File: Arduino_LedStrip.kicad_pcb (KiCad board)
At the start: 2 copper layers, 52 x 71 mm, 26 parts, among them J1 Conn_L, J2 Conn_R, J3 LED0, J4 LED1, J5 LED_WS2812B, J6 Barrel_Jack, Q1 IRFZ44N, Q2 IRFZ44N, Q3 IRFZ44N, Q4 IRFZ44N, Q5 IRFZ44N, Q6 IRFZ44N, SW1 SW_Push, SW2 SW_Push, U1 TSOP4838

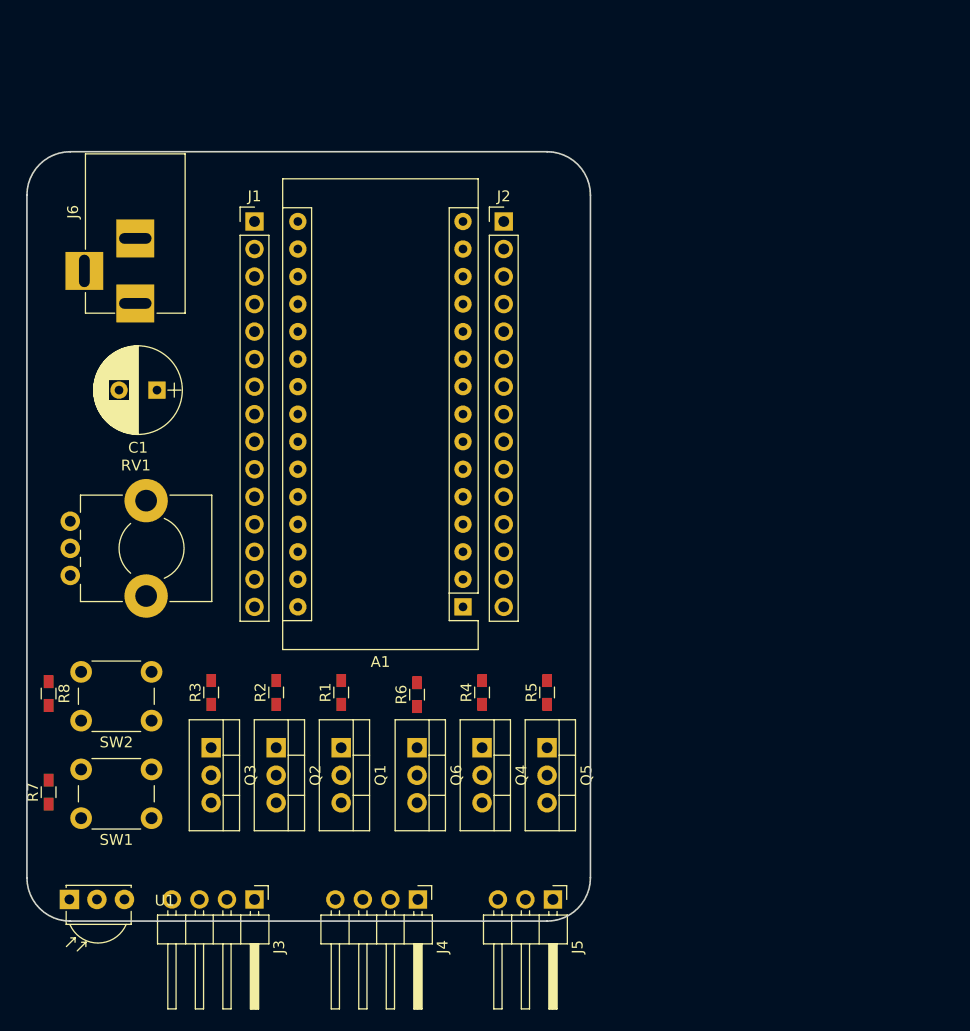
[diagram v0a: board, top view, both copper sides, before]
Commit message: Routing PCB
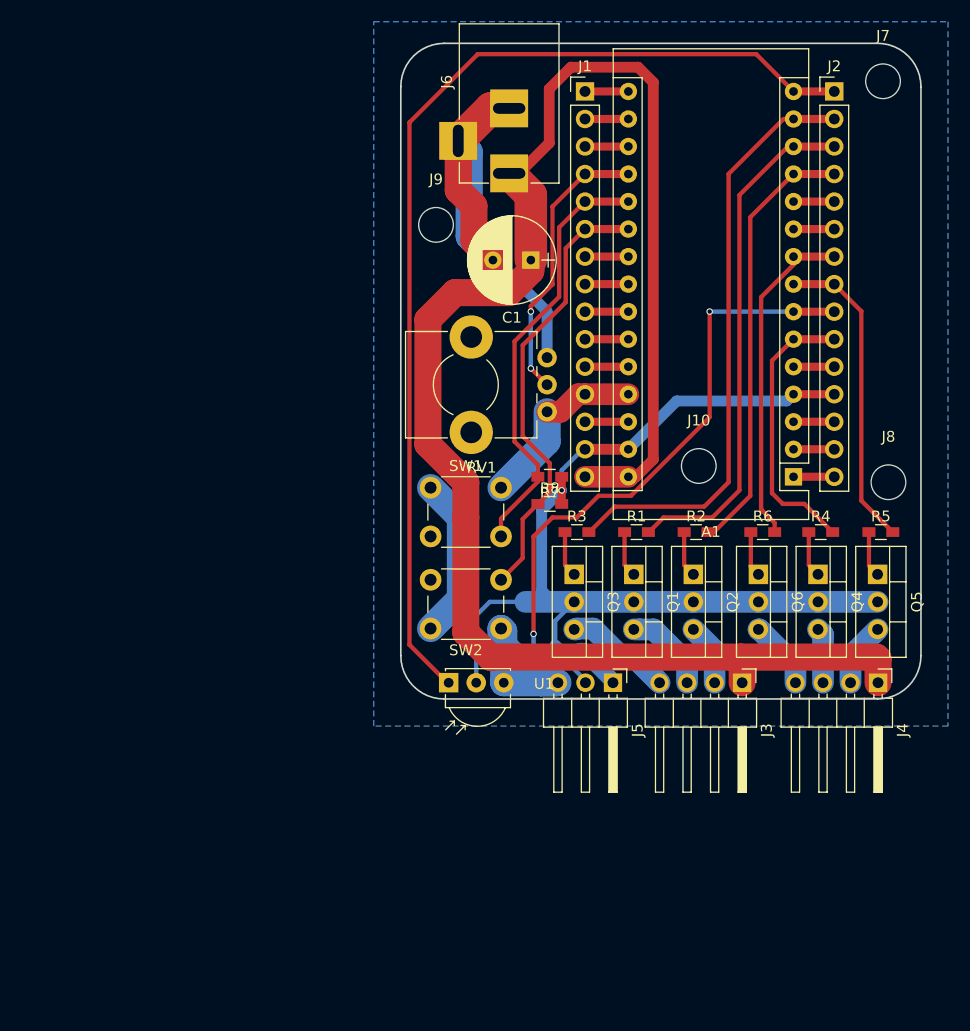
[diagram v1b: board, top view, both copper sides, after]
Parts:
- added J10: Screw_Terminal_01x01, Mounting_Holes:MountingHole_3.2mm_M3, F.Cu at (150.0, 91.0)
- added J7: Screw_Terminal_01x01, Mounting_Holes:MountingHole_3.2mm_M3, F.Cu at (167.0, 55.5)
- added J8: Screw_Terminal_01x01, Mounting_Holes:MountingHole_3.2mm_M3, F.Cu at (167.5, 92.5)
- added J9: Screw_Terminal_01x01, Mounting_Holes:MountingHole_3.2mm_M3, F.Cu at (125.8, 68.8)
- moved R7 54.6 mm to (136.2, 92.0), turned to 180 degrees
- moved R8 49.5 mm to (136.2, 94.5), turned to 0 degrees
- moved J3 49.2 mm to (154.0, 111.0)
- moved RV1 48.4 mm to (136.0, 81.0), turned to 180 degrees
- moved J4 46.9 mm to (166.5, 111.0)
- moved Q2 41.7 mm to (149.5, 101.0)
- moved R2 41.5 mm to (149.8, 97.1), turned to 0 degrees
- moved U1 40.3 mm to (126.9, 111.0)
- moved SW1 39.9 mm to (125.2, 93.0), turned to 0 degrees
- moved Q3 37.1 mm to (138.5, 101.0)
- moved R3 36.9 mm to (138.8, 97.1), turned to 0 degrees
- moved C1 36.5 mm to (134.5, 72.0)
- moved J6 36.5 mm to (132.5, 64.0)
- moved Q6 35.3 mm to (155.5, 101.0)
- moved R6 35.3 mm to (155.9, 97.1), turned to 0 degrees
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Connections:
- A1 pad 12: /ar_LED0_R -> /ar_LED0_G
- A1 pad 13: /ar_LED0_G -> /ar_LED0_R
- J2 pad 3: /ar_LED0_G -> /ar_LED0_R
- J2 pad 4: /ar_LED0_R -> /ar_LED0_G
- J5 pad 1: +5V -> GND
- J5 pad 3: GND -> +5V
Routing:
- net +12V: track 0.00 -> 166.6 mm
- net GND: track 0.00 -> 150.9 mm, vias 0 -> 1
- net /ar_IR: track 0.00 -> 96.5 mm
- net /ar_Din_LEDWS: track 0.00 -> 58.7 mm, vias 0 -> 2
- net /ar_LED0_B: track 0.00 -> 55.1 mm
- net +5V: track 0.00 -> 50.3 mm
- net /ar_LED0_R: track 0.00 -> 47.9 mm
- net /ar_A2_D16: track 0.00 -> 41.6 mm
- net /ar_LED0_G: track 0.00 -> 40.4 mm
- net /ar_A1_D15: track 0.00 -> 39.9 mm
- net /ar_LED1_B: track 0.00 -> 30.9 mm
- net /ar_LED1_G: track 0.00 -> 28.9 mm
- net /ar_A0_Pot: track 0.00 -> 26.1 mm, vias 0 -> 2
- net /ar_LED1_R: track 0.00 -> 25.9 mm
- net /LED0_B: track 0.00 -> 9.98 mm
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- added copper zone on B.Cu, net GND
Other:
- board size 52 x 71 mm -> 48 x 60.5 mm
- net class Default: clearance 0.2 -> 0.21
- rule trace_clearance: 0.2 -> 0.21

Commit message: Update routing.
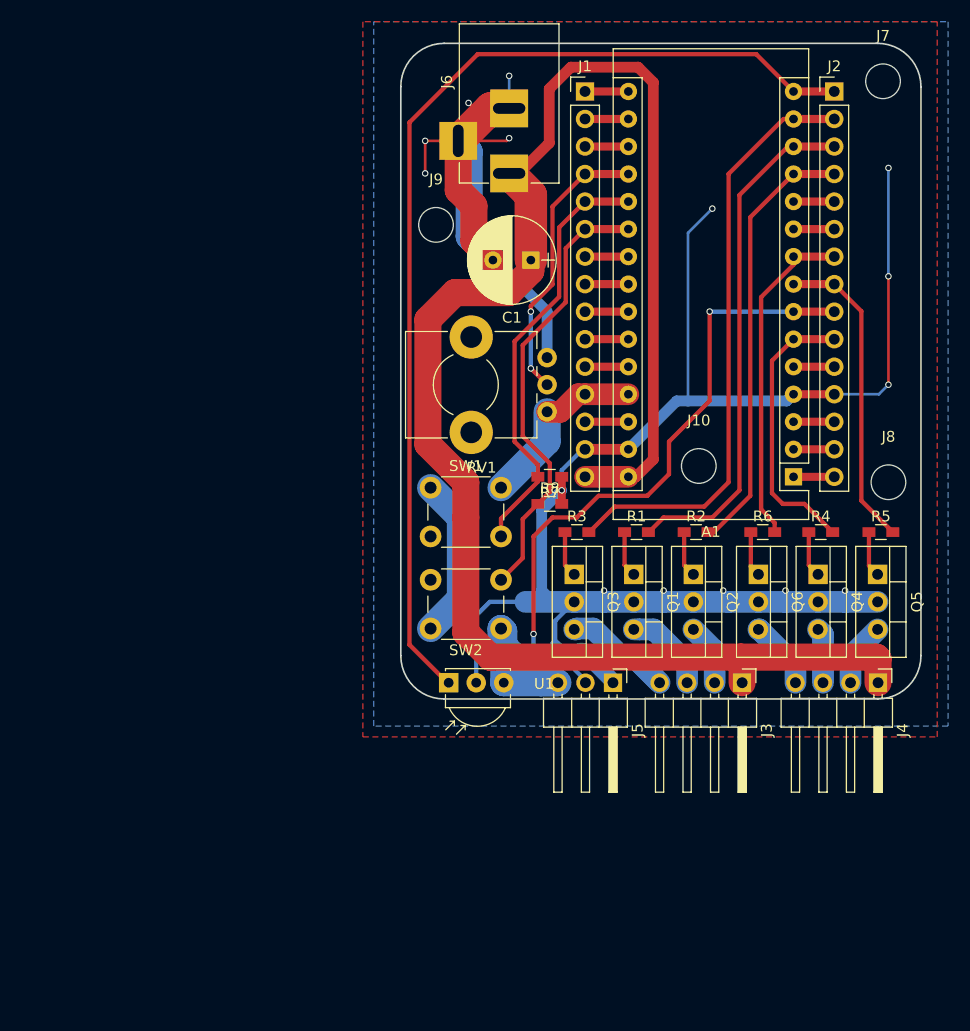
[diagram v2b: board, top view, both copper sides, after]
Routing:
- net GND: track 150.9 -> 218.2 mm, vias 1 -> 15
- net /ar_Din_LEDWS: track 58.7 -> 59.5 mm
- added copper zone on F.Cu, net GND
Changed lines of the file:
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@@
     (links 83)
     (no_connects 4)
-    (area 122.424999 51.924999 170.575001 112.575001)
+    (area 117.111428 40.3 183.35 121.785001)
     (thickness 1.6)
     (drawings 10)
-    (tracks 233)
+    (tracks 274)
     (zones 0)
     (modules 30)
@@
   )
   (setup
-    (last_trace_width 1)
+    (last_trace_width 0.25)
     (user_trace_width 0.4)
     (user_trace_width 0.75)
@@
     (user_trace_width 3)
     (trace_clearance 0.21)
-    (zone_clearance 0.508)
+    (zone_clearance 0.75)
     (zone_45_only no)
     (trace_min 0.2)
@@
   (segment (start 134.5 82) (end 136 83.5) (width 0.4) (layer F.Cu) (net 6))
   (segment (start 143.5 64.06) (end 139.5 64.06) (width 0.75) (layer F.Cu) (net 6))
+  (segment (start 127.8 61) (end 132.25 61) (width 0.25) (layer F.Cu) (net 7))
+  (segment (start 132.25 61) (end 132.5 60.75) (width 0.25) (layer F.Cu) (net 7))
+  (via (at 132.5 60.75) (size 0.6) (drill 0.4) (layers F.Cu B.Cu) (net 7))
+  (segment (start 124.75 61) (end 124.75 64) (width 0.25) (layer F.Cu) (net 7))
+  (via (at 124.75 64) (size 0.6) (drill 0.4) (layers F.Cu B.Cu) (net 7))
+  (segment (start 132.5 58) (end 129.25 58) (width 0.25) (layer F.Cu) (net 7))
+  (segment (start 129.25 58) (end 128.75 57.5) (width 0.25) (layer F.Cu) (net 7))
+  (via (at 128.75 57.5) (size 0.6) (drill 0.4) (layers F.Cu B.Cu) (net 7))
+  (segment (start 132.5 58) (end 132.5 55) (width 0.25) (layer B.Cu) (net 7))
+  (via (at 132.5 55) (size 0.6) (drill 0.4) (layers F.Cu B.Cu) (net 7))
+  (segment (start 127.8 61) (end 124.75 61) (width 0.25) (layer F.Cu) (net 7))
+  (via (at 124.75 61) (size 0.6) (drill 0.4) (layers F.Cu B.Cu) (net 7))
+  (segment (start 127.8 61) (end 127.8 65.55) (width 2.5) (layer F.Cu) (net 7))
+  (segment (start 149 85) (end 158.12 85) (width 1) (layer B.Cu) (net 7))
+  (segment (start 147.96 85) (end 149 85) (width 1) (layer B.Cu) (net 7))
+  (segment (start 149 85) (end 149 69.5) (width 0.25) (layer B.Cu) (net 7))
+  (segment (start 149 69.5) (end 151.25 67.25) (width 0.25) (layer B.Cu) (net 7))
+  (via (at 151.25 67.25) (size 0.6) (drill 0.4) (layers F.Cu B.Cu) (net 7))
+  (segment (start 167.5 73.5) (end 167.5 63.5) (width 0.25) (layer B.Cu) (net 7))
+  (via (at 167.5 63.5) (size 0.6) (drill 0.4) (layers F.Cu B.Cu) (net 7))
+  (segment (start 167.5 83.5) (end 167.5 73.5) (width 0.25) (layer F.Cu) (net 7))
+  (via (at 167.5 73.5) (size 0.6) (drill 0.4) (layers F.Cu B.Cu) (net 7))
+  (segment (start 162.5 84.38) (end 166.62 84.38) (width 0.25) (layer B.Cu) (net 7))
+  (via (at 167.5 83.5) (size 0.6) (drill 0.4) (layers F.Cu B.Cu) (net 7))
+  (segment (start 166.62 84.38) (end 167.5 83.5) (width 0.25) (layer B.Cu) (net 7))
+  (segment (start 163.5 103.54) (end 166.5 103.54) (width 2) (layer B.Cu) (net 7))
+  (segment (start 161 103.54) (end 163.5 103.54) (width 2) (layer B.Cu) (net 7))
+  (segment (start 163.5 103.54) (end 163.5 102.5) (width 0.25) (layer B.Cu) (net 7))
+  (via (at 163.5 102.5) (size 0.6) (drill 0.4) (layers F.Cu B.Cu) (net 7))
+  (segment (start 158 103.54) (end 161 103.54) (width 2) (layer B.Cu) (net 7))
+  (segment (start 155.5 103.54) (end 158 103.54) (width 2) (layer B.Cu) (net 7))
+  (via (at 158 102.5) (size 0.6) (drill 0.4) (layers F.Cu B.Cu) (net 7))
+  (segment (start 158 103.54) (end 158 102.5) (width 0.25) (layer B.Cu) (net 7))
+  (segment (start 152.75 103.54) (end 152.25 103.04) (width 0.25) (layer B.Cu) (net 7))
+  (segment (start 152.25 103.04) (end 152.25 102.5) (width 0.25) (layer B.Cu) (net 7))
+  (via (at 152.25 102.5) (size 0.6) (drill 0.4) (layers F.Cu B.Cu) (net 7))
+  (segment (start 146.75 103.54) (end 146.75 102.5) (width 0.25) (layer B.Cu) (net 7))
+  (via (at 146.75 102.5) (size 0.6) (drill 0.4) (layers F.Cu B.Cu) (net 7))
+  (segment (start 152.75 103.54) (end 155.5 103.54) (width 2) (layer B.Cu) (net 7))
+  (segment (start 149.5 103.54) (end 152.75 103.54) (width 2) (layer B.Cu) (net 7))
+  (segment (start 146.75 103.54) (end 149.5 103.54) (width 2) (layer B.Cu) (net 7))
+  (segment (start 144 103.54) (end 146.75 103.54) (width 2) (layer B.Cu) (net 7))
+  (segment (start 141.25 103.54) (end 144 103.54) (width 2) (layer B.Cu) (net 7))
+  (segment (start 141.25 103.54) (end 141.25 102.5) (width 0.25) (layer B.Cu) (net 7))
+  (segment (start 138.5 103.54) (end 141.25 103.54) (width 2) (layer B.Cu) (net 7))
+  (via (at 141.25 102.5) (size 0.6) (drill 0.4) (layers F.Cu B.Cu) (net 7))
   (segment (start 139.292857 108.074055) (end 137.324055 108.074055) (width 1) (layer B.Cu) (net 7))
   (segment (start 137.324055 108.074055) (end 136.75 107.5) (width 1) (layer B.Cu) (net 7))
@@
   (segment (start 136.54 103.54) (end 138.5 103.54) (width 1) (layer B.Cu) (net 7))
   (segment (start 143.5 89.46) (end 147.96 85) (width 1) (layer B.Cu) (net 7))
-  (segment (start 147.96 85) (end 158.12 85) (width 1) (layer B.Cu) (net 7))
   (segment (start 158.12 85) (end 158.74 84.38) (width 1) (layer B.Cu) (net 7))
   (segment (start 136 81) (end 136 76.755198) (width 1) (layer B.Cu) (net 7))
@@
   (segment (start 131.244802 72) (end 131 72) (width 1) (layer B.Cu) (net 7))
   (segment (start 138.5 103.54) (end 134 103.54) (width 2) (layer B.Cu) (net 7))
-  (segment (start 161 103.54) (end 166.5 103.54) (width 2) (layer B.Cu) (net 7))
-  (segment (start 155.5 103.54) (end 161 103.54) (width 2) (layer B.Cu) (net 7))
-  (segment (start 149.5 103.54) (end 155.5 103.54) (width 2) (layer B.Cu) (net 7))
-  (segment (start 144 103.54) (end 149.5 103.54) (width 2) (layer B.Cu) (net 7))
-  (segment (start 138.5 103.54) (end 144 103.54) (width 2) (layer B.Cu) (net 7))
   (segment (start 136.75 107.5) (end 136.75 105.29) (width 0.4) (layer B.Cu) (net 7))
   (segment (start 136.75 105.29) (end 138.5 103.54) (width 0.4) (layer B.Cu) (net 7))
   (segment (start 129.46 111) (end 129.5 110.96) (width 0.4) (layer B.Cu) (net 7))
-  (segment (start 127.8 61) (end 127.8 65.55) (width 2.5) (layer F.Cu) (net 7))
   (segment (start 127.8 65.55) (end 129.25 67) (width 2.5) (layer F.Cu) (net 7))
   (segment (start 129.25 67) (end 129.25 70.25) (width 2.5) (layer F.Cu) (net 7))
@@
   (segment (start 139.54 111) (end 139.5 111) (width 0.4) (layer B.Cu) (net 13))
   (segment (start 139.5 111) (end 139.5 110.75) (width 0.4) (layer B.Cu) (net 13))
-  (segment (start 137.75 109) (end 135.75 109) (width 0.4) (layer B.Cu) (net 13))
   (segment (start 139.5 110.75) (end 137.75 109) (width 0.4) (layer B.Cu) (net 13))
-  (segment (start 135.75 109) (end 134.75 108) (width 0.4) (layer B.Cu) (net 13))
-  (segment (start 134.75 108) (end 134.75 106.5) (width 0.4) (layer B.Cu) (net 13))
+  (segment (start 137.75 109) (end 136 109) (width 0.4) (layer B.Cu) (net 13))
+  (segment (start 136 109) (end 134.75 107.75) (width 0.4) (layer B.Cu) (net 13))
+  (segment (start 134.75 107.75) (end 134.75 106.5) (width 0.4) (layer B.Cu) (net 13))
+  (segment (start 151 76.75) (end 151 85) (width 0.4) (layer F.Cu) (net 13))
+  (segment (start 151 85) (end 147.25 88.75) (width 0.4) (layer F.Cu) (net 13))
+  (segment (start 147.25 88.75) (end 147.25 91.75) (width 0.4) (layer F.Cu) (net 13))
+  (segment (start 147.25 91.75) (end 145.25 93.75) (width 0.4) (layer F.Cu) (net 13))
+  (segment (start 145.25 93.75) (end 140.75 93.75) (width 0.4) (layer F.Cu) (net 13))
+  (segment (start 138.75 95.75) (end 136.5 95.75) (width 0.4) (layer F.Cu) (net 13))
+  (segment (start 140.75 93.75) (end 138.75 95.75) (width 0.4) (layer F.Cu) (net 13))
+  (segment (start 136.5 95.75) (end 134.75 97.5) (width 0.4) (layer F.Cu) (net 13))
   (segment (start 134.75 97.5) (end 134.75 106.5) (width 0.4) (layer F.Cu) (net 13))
-  (segment (start 136.5 95.75) (end 134.75 97.5) (width 0.4) (layer F.Cu) (net 13))
-  (segment (start 140.75 93.75) (end 138.75 95.75) (width 0.4) (layer F.Cu) (net 13))
-  (segment (start 143.744055 93.75) (end 140.75 93.75) (width 0.4) (layer F.Cu) (net 13))
-  (segment (start 151 86.494055) (end 143.744055 93.75) (width 0.4) (layer F.Cu) (net 13))
-  (segment (start 138.75 95.75) (end 136.5 95.75) (width 0.4) (layer F.Cu) (net 13))
-  (segment (start 151 76.75) (end 151 86.494055) (width 0.4) (layer F.Cu) (net 13))
   (via (at 134.75 106.5) (size 0.6) (drill 0.4) (layers F.Cu B.Cu) (net 13))
   (segment (start 158.74 76.76) (end 151.01 76.76) (width 0.4) (layer B.Cu) (net 13))
@@
       )
     )
+  )
+  (zone (net 7) (net_name GND) (layer F.Cu) (hatch edge 0.508)
+    (connect_pads (clearance 0.75))
+    (min_thickness 0.254)
+    (fill yes (arc_segments 16) (thermal_gap 0.508) (thermal_bridge_width 0.508))
+    (polygon
+      (pts
+        (xy 119 116) (xy 172 116) (xy 172 50) (xy 119 50)
+      )
+    )
